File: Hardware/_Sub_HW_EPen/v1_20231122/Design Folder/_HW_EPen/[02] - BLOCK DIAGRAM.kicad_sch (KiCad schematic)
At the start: 0 parts

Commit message: _HW_EPen is ready to be worked for layout
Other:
- title: EPen -> _HW_EPen
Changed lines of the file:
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@@
   (paper "B")
   (title_block
-    (title "EPen")
+    (title "_HW_EPen")
     (date "2023-11-27")
     (rev "v1.0")
     (company "mend0z0")
     (comment 1 "v1.0")
-    (comment 2 "PRELIMINARY")
+    (comment 2 "CHECKED")
     (comment 4 "_BOM_EPen.html")
     (comment 5 "_HW_EPen.pcb")
     (comment 6 "_GBR_EPen.zip")
     (comment 7 "_BOM_EPen.html")
+    (comment 8 "N/A")
     (comment 9 "First Release")
   )

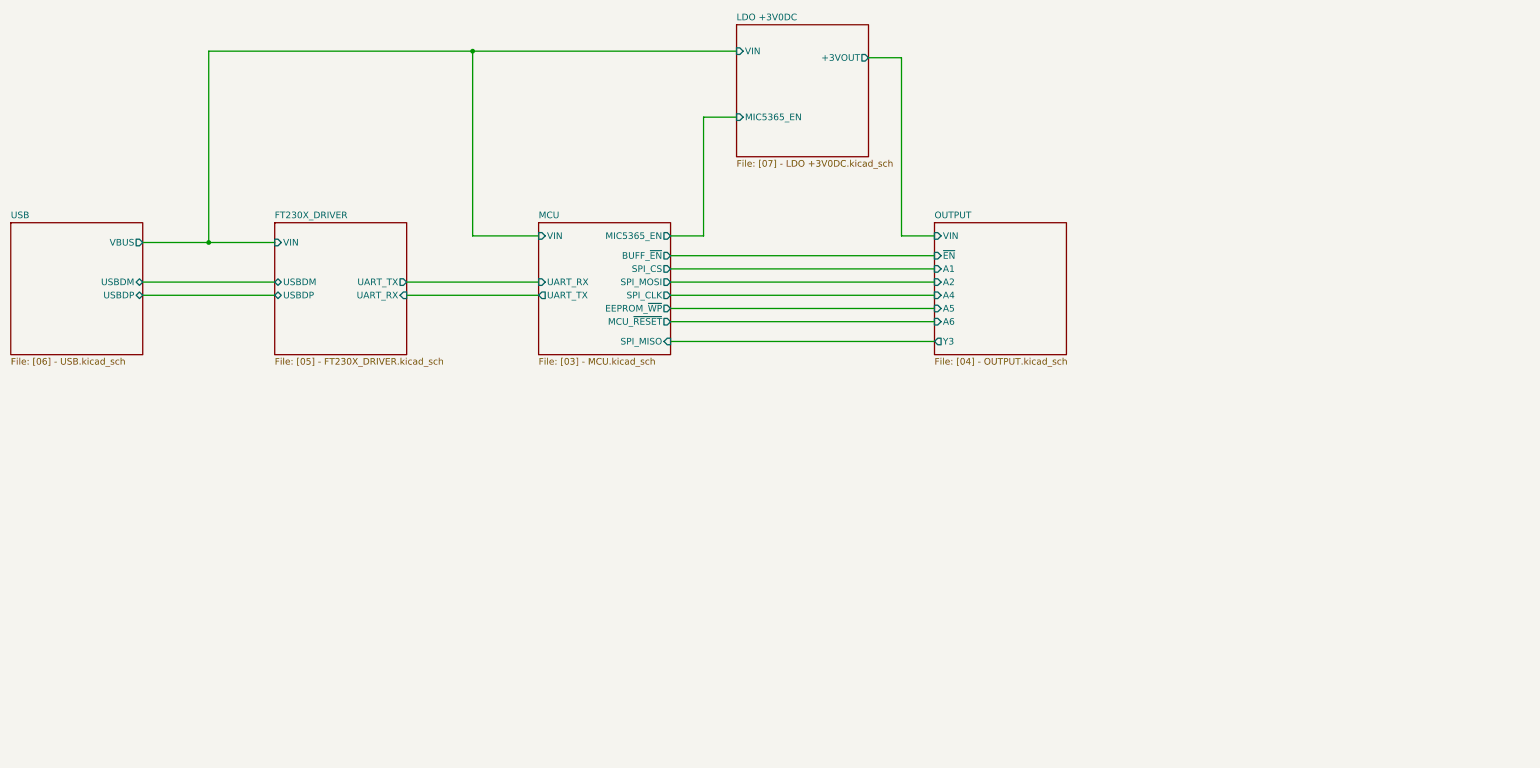
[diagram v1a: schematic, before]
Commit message: Updating file templates and structures...
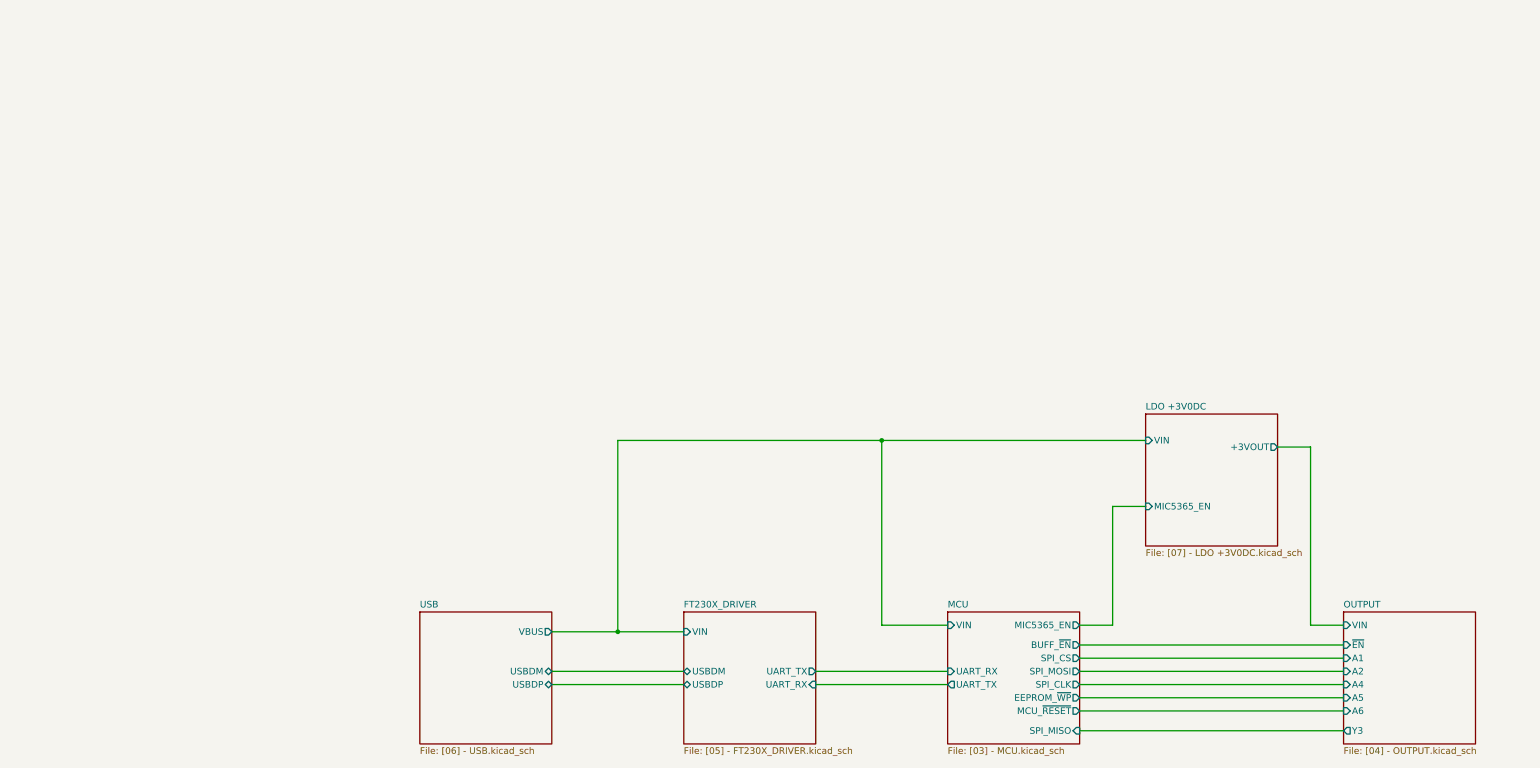
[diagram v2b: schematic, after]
